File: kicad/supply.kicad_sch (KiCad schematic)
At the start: 50 parts, among them J8 Screw_Terminal_01x03, U14 TMUX6123, U17 TMUX6123, U19 L7815, U23 L7915, U6 LM2937-5, U9 LM317_TO-252

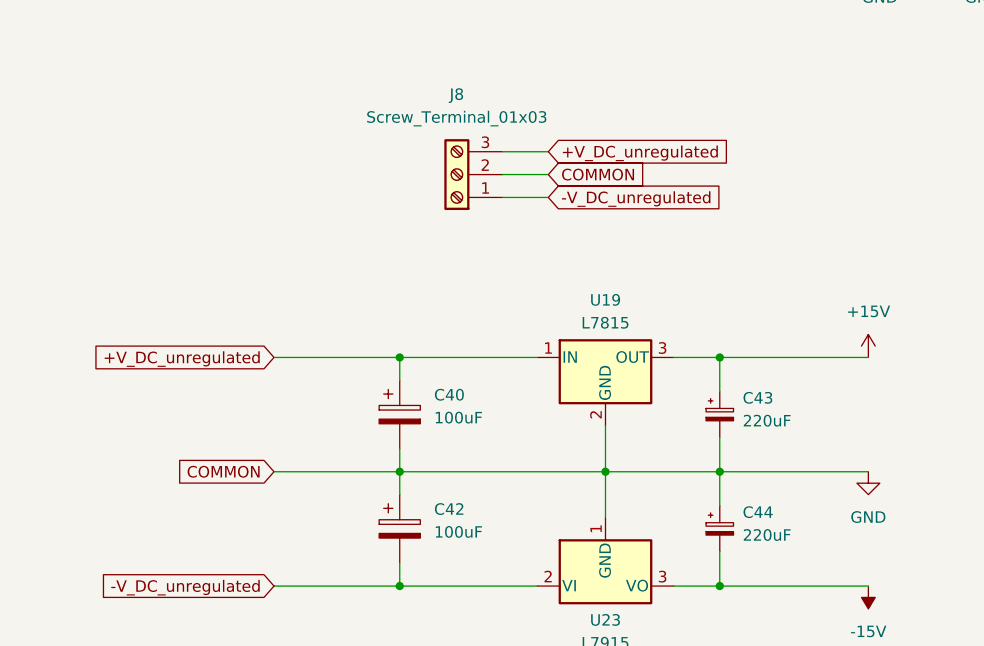
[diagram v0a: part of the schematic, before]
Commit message: Final Schematic, Reworking PCB pt 1
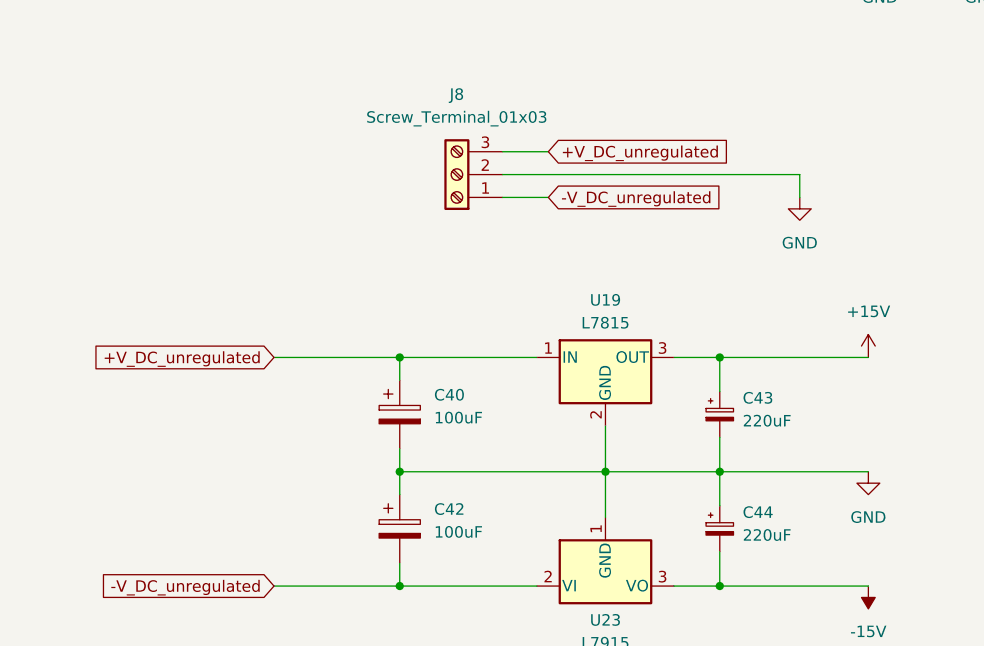
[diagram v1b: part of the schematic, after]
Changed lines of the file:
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@@
 	(wire
 		(pts
-			(xy 72.39 168.91) (xy 86.36 168.91)
-		)
-		(stroke
-			(width 0)
-			(type default)
-		)
-	)
-	(wire
-		(pts
 			(xy 176.53 62.865) (xy 176.53 66.675)
 		)
@@
 	(wire
 		(pts
-			(xy 97.79 135.89) (xy 102.87 135.89)
-		)
-		(stroke
-			(width 0)
-			(type default)
-		)
-	)
-	(wire
-		(pts
 			(xy 160.655 52.07) (xy 176.53 52.07)
 		)
@@
 	(wire
 		(pts
+			(xy 130.81 138.43) (xy 130.81 135.89)
+		)
+		(stroke
+			(width 0)
+			(type default)
+		)
+	)
+	(wire
+		(pts
 			(xy 226.06 112.395) (xy 226.06 113.03)
 		)
@@
 	(wire
 		(pts
+			(xy 130.81 135.89) (xy 97.79 135.89)
+		)
+		(stroke
+			(width 0)
+			(type default)
+		)
+	)
+	(wire
+		(pts
 			(xy 78.74 49.53) (xy 78.74 52.07)
 		)
@@
 		)
 	)
-	(global_label "COMMON"
-		(shape input)
-		(at 72.39 168.91 180)
-		(fields_autoplaced yes)
-		(effects
-			(font
-				(size 1.27 1.27)
-			)
-			(justify right)
-		)
-		(property "Intersheetrefs" "${INTERSHEET_REFS}"
-			(at 61.2405 168.91 0)
-			(effects
-				(font
-					(size 1.27 1.27)
-				)
-				(justify right)
-				(hide yes)
-			)
-		)
-	)
 	(global_label "+V_DC_unregulated"
 		(shape input)
@@
 		)
 	)
-	(global_label "COMMON"
-		(shape input)
-		(at 102.87 135.89 0)
-		(fields_autoplaced yes)
-		(effects
-			(font
-				(size 1.27 1.27)
-			)
-			(justify left)
-		)
-		(property "Intersheetrefs" "${INTERSHEET_REFS}"
-			(at 114.0195 135.89 0)
-			(effects
-				(font
-					(size 1.27 1.27)
-				)
-				(justify left)
-				(hide yes)
-			)
-		)
-	)
 	(global_label "-V_DC_unregulated"
 		(shape input)
@@
 					(unit 1)
 				)
+			)
+		)
+	)
+	(symbol
+		(lib_id "power:GND")
+		(at 130.81 138.43 0)
+		(unit 1)
+		(exclude_from_sim no)
+		(in_bom yes)
+		(on_board yes)
+		(dnp no)
+		(fields_autoplaced yes)
+		(property "Reference" "#PWR081"
+			(at 130.81 144.78 0)
+			(effects
+				(font
+					(size 1.27 1.27)
+				)
+				(hide yes)
+			)
+		)
+		(property "Value" "GND"
+			(at 130.81 143.51 0)
+			(effects
+				(font
+					(size 1.27 1.27)
+				)
+			)
+		)
+		(property "Footprint" ""
+			(at 130.81 138.43 0)
+			(effects
+				(font
+					(size 1.27 1.27)
+				)
+				(hide yes)
+			)
+		)
+		(property "Datasheet" ""
+			(at 130.81 138.43 0)
+			(effects
+				(font
+					(size 1.27 1.27)
+				)
+				(hide yes)
+			)
+		)
+		(property "Description" ""
+			(at 130.81 138.43 0)
+			(effects
+				(font
+					(size 1.27 1.27)
+				)
+				(hide yes)
+			)
+		)
+		(pin "1"
+		)
+		(instances
+			(project "intensity_pi"
+				(path "/3a3d7bcb-6fa5-41ef-9ea1-6d4ab7c492fd/a04c5785-e230-4149-bf27-97ee4701c201"
+					(reference "#PWR081")
+					(unit 1)
+				)
